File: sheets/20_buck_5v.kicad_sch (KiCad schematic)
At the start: 12 parts, among them U201 LMR38010SQDDARQ1

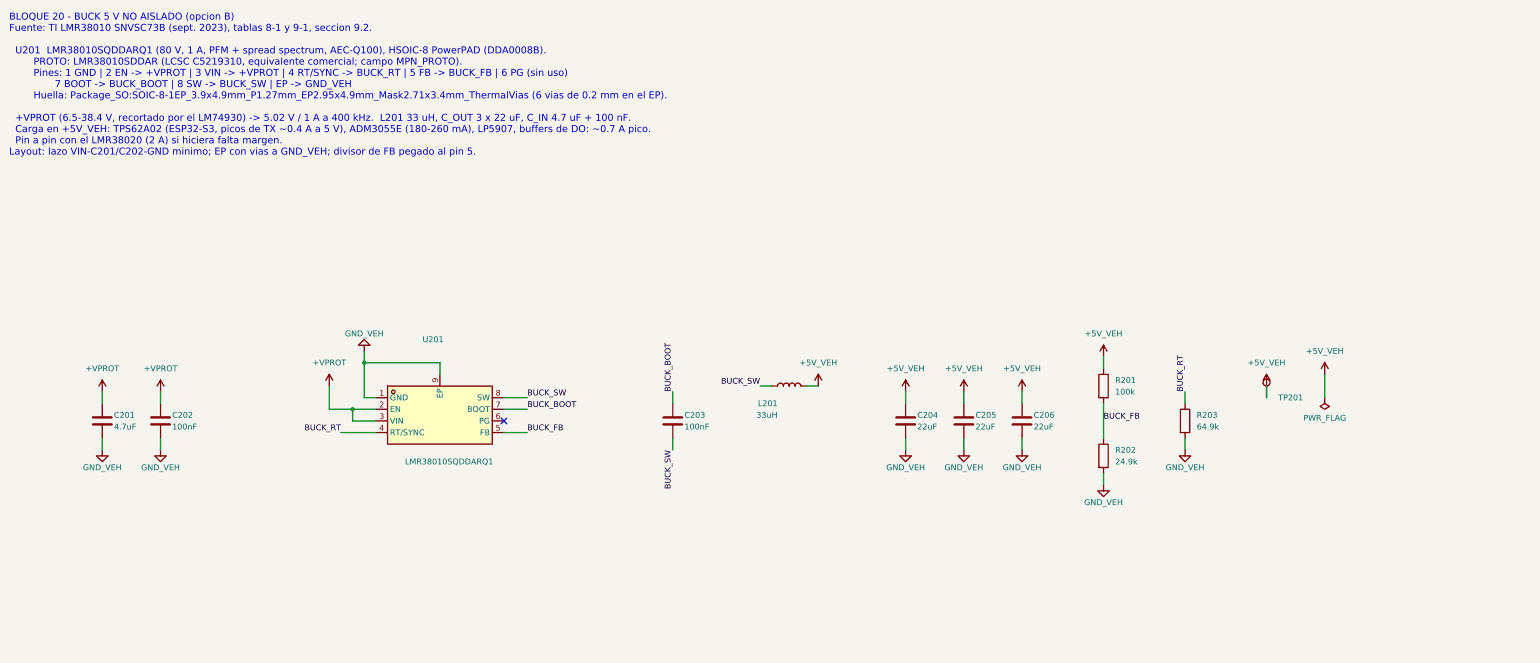
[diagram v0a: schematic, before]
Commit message: update pcb layout
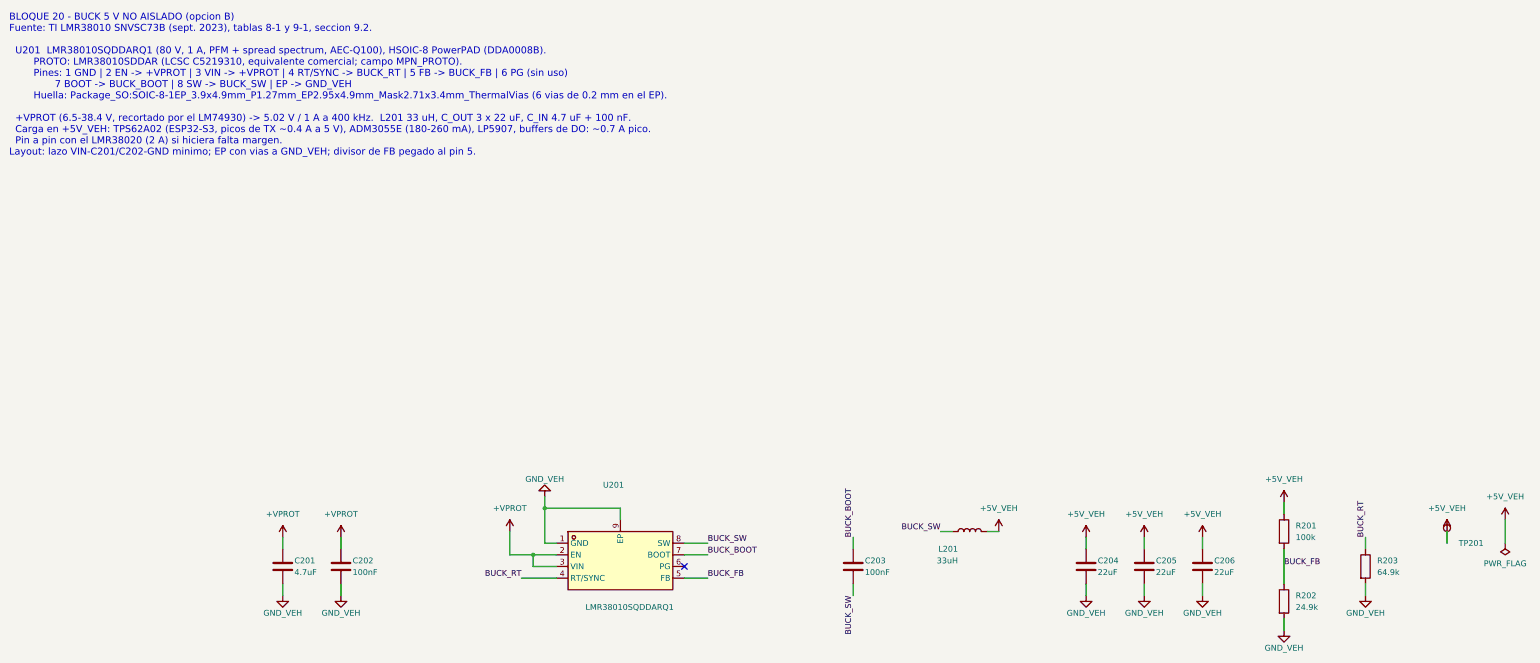
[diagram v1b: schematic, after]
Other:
- moved on the sheet: C201, C202, C203, C204, C205, C206, L201, R201, R202, R203, TP201, U201
